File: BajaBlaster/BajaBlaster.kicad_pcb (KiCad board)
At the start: 4 copper layers, 64.5 x 51 mm, 42 parts, among them J201 Conn_01x02_Pin, J301 Conn_01x06_Socket, J501 Conn_01x06_Pin, J502 INTERBOARD, J503 Conn_01x04_Pin, SW301 SW_Push, SW302 SW_Push, U201 AP2112K-3.3, U202 TPS562200, U301 ESP32-WROOM-32, U302 MPU-6050, U501 TCAN330

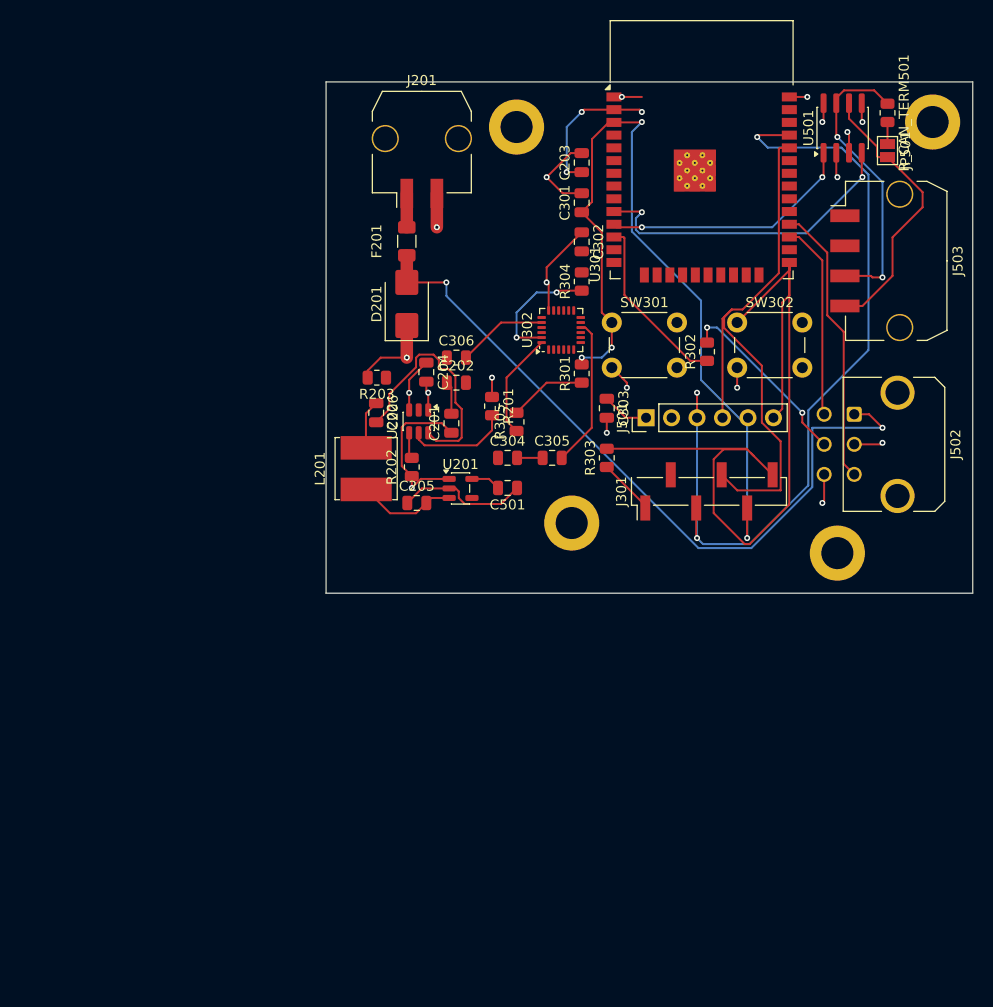
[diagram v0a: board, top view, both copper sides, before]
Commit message: fixed andrews layout
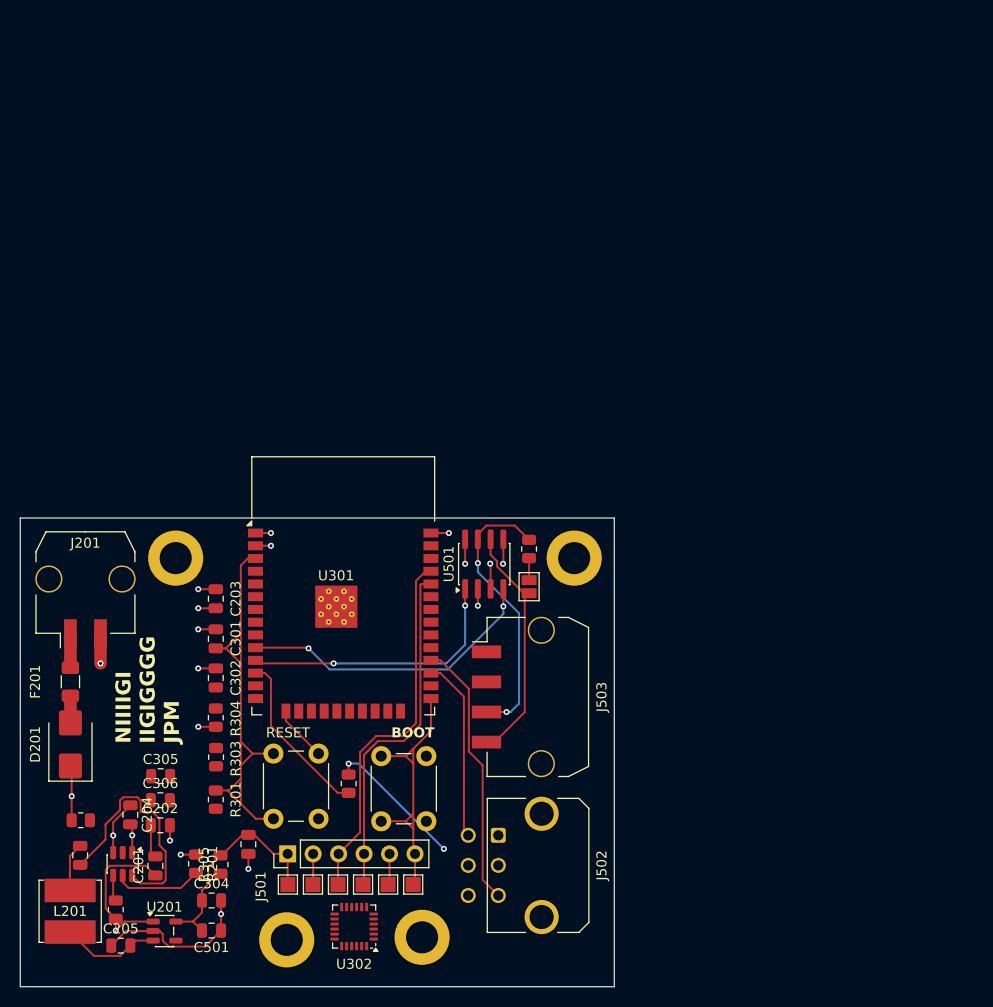
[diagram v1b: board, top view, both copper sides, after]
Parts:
- removed J301: Conn_01x06_Socket, Connector_PinHeader_2.54mm:PinHeader_1x06_P2.54mm_Vertical_SMD_Pin1Left
- added REF**: TestPoint_Pad_1.5x1.5mm, TestPoint:TestPoint_Pad_1.5x1.5mm, F.Cu at (51.7, 111.6)
- added REF**: TestPoint_Pad_1.5x1.5mm, TestPoint:TestPoint_Pad_1.5x1.5mm, F.Cu at (59.2, 111.6)
- added REF**: TestPoint_Pad_1.5x1.5mm, TestPoint:TestPoint_Pad_1.5x1.5mm, F.Cu at (56.7, 111.6)
- added REF**: TestPoint_Pad_1.5x1.5mm, TestPoint:TestPoint_Pad_1.5x1.5mm, F.Cu at (54.2, 111.6)
- added REF**: TestPoint_Pad_1.5x1.5mm, TestPoint:TestPoint_Pad_1.5x1.5mm, F.Cu at (61.7, 111.6)
- added REF**: TestPoint_Pad_1.5x1.5mm, TestPoint:TestPoint_Pad_1.5x1.5mm, F.Cu at (64.2, 111.6)
- moved U302 63.0 mm to (58.3, 115.8), turned to 180 degrees
- moved SW302 61.1 mm to (61.0, 105.2), turned to 90 degrees
- moved SW301 59.9 mm to (50.2, 105.0), turned to 90 degrees
- moved C203 56.8 mm to (44.5, 83.0)
- moved C301 56.8 mm to (44.5, 87.0)
- moved C302 56.8 mm to (44.5, 91.0)
- moved R304 56.8 mm to (44.5, 94.9)
- moved REF** 56.4 mm to (65.1, 116.8)
- moved C303 56.3 mm to (47.8, 107.5)
- moved J501 56.3 mm to (51.7, 108.5)
- moved REF** 56.3 mm to (80.2, 79.0)
- moved R_CAN_TERM501 56.3 mm to (75.8, 78.1)
- moved U501 56.3 mm to (71.3, 79.6)
- moved J503 56.3 mm to (76.6, 92.8)
- moved JP501 56.3 mm to (75.8, 81.8)
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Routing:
- net +12V: track 81.1 -> 11.2 mm, vias 4 -> 3
- net /COMMS/IO0: track 86.0 -> 29.3 mm
- net /COMMS/U0TXD: track 83.2 -> 37.0 mm, vias 3 -> 0
- net /COMMS/ESP32_EN: track 81.9 -> 48.9 mm, vias 4 -> 0
- net /COMMS/U0RXD: track 58.1 -> 36.6 mm
- net GND: track 73.7 -> 56.1 mm, vias 15 -> 13
- net Net-(U302-REGOUT): track 15.0 -> 0.00 mm
- net Net-(U302-SDA): track 10.7 -> 0.00 mm
- net Net-(U302-SCL): track 12.4 -> 1.75 mm, vias 2 -> 1
- net +3V3: track 37.5 -> 28.5 mm, vias 4 -> 3
- net Net-(U302-CPOUT): track 9.00 -> 0.00 mm
- net /COMMS/SYNC: track 18.6 -> 14.5 mm
- net /COMMS/CANL: track 28.1 -> 24.4 mm
- net /COMMS/CAN_RX: track 32.3 -> 30.4 mm
- net /COMMS/CAN_TX: track 25.5 -> 27.4 mm
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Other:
- board size 64.5 x 51 mm -> 59.2 x 46.8 mm
- board text added: "BOOT"
- board text added: "NIIIIGI IIGIGGGG JPM"
- board text added: "RESET"
